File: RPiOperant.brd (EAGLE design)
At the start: 136 x 100 mm, 69 parts, among them IC1 74LS14N, IC2 74LS14N, IC3 MCP3008, J1 USB_B_PTH, J2 POWER_JACK, J3 POWER_JACK, J4 USB_B_PTH, J5 1X2-3.5MM, J6 1X2-3.5MM

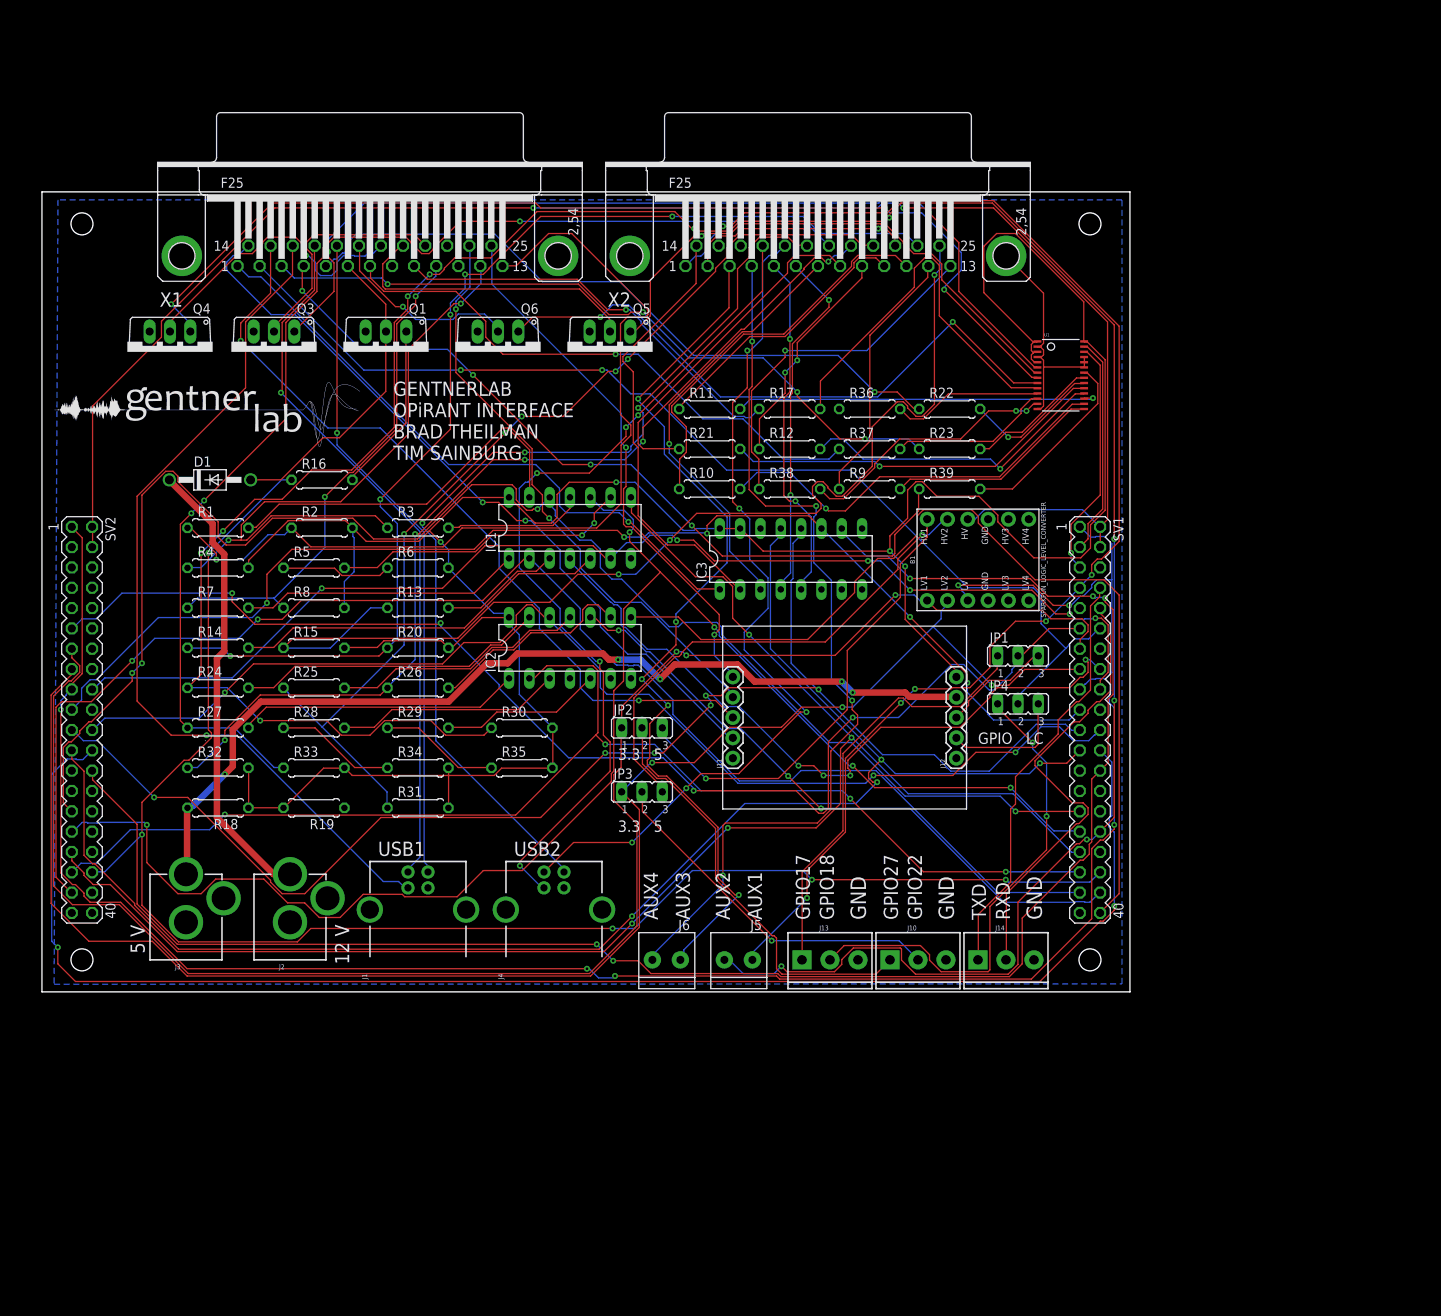
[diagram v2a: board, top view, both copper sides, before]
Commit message: alternate
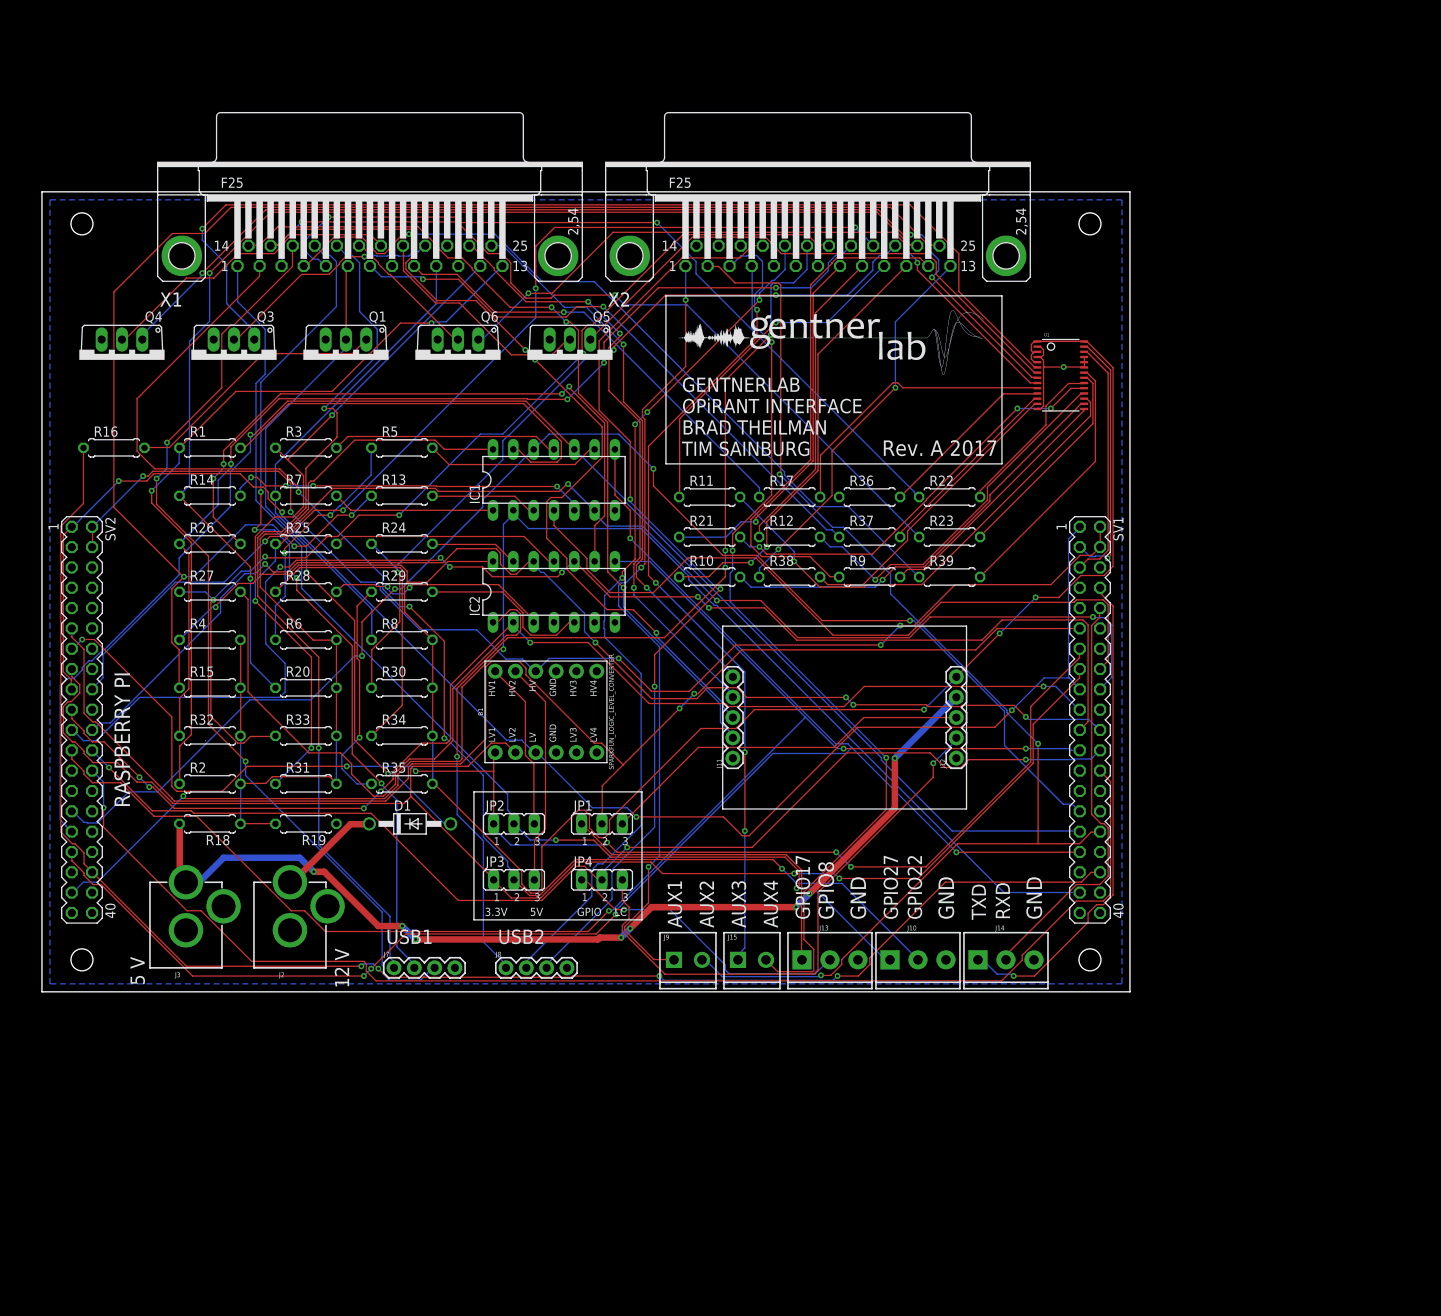
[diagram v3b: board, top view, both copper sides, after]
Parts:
- removed IC3: MCP3008, adafruit:DIL16
- removed J1, J4: USB_B_PTH, SparkFun-Connectors:USB-B-PTH
- removed J5, J6: 1X2-3.5MM, adafruit:1X2-3.5MM
- added J15, J9: (no value), SparkFun-Connectors:SCREWTERMINAL-3.5MM-2
- added J7, J8: (no value), SparkFun-Connectors:1X04
- moved B1 57.2 mm to (63.0, 35.0)
- moved JP4 56.5 mm to (70.0, 14.0)
- moved JP1 56.1 mm to (70.0, 21.0)
- moved D1 49.7 mm to (46.0, 21.0)
- moved R2 34.9 mm to (21.0, 26.0)
- moved R26 31.6 mm to (21.0, 56.0)
- moved R24 29.2 mm to (45.0, 56.0)
- moved R16 26.3 mm to (9.00, 68.0)
- moved JP2 20.0 mm to (59.0, 21.0)
- moved JP3 19.4 mm to (59.0, 14.0)
- moved R14 19.0 mm to (21.0, 62.0)
- moved R5 18.6 mm to (45.0, 68.0)
- moved R25 18.0 mm to (33.0, 56.0)
- moved R7 17.8 mm to (33.0, 62.0)
- moved R3 17.2 mm to (33.0, 68.0)
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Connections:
- removed net ADC0: IC3.1, X1.1
- removed net ADC1: IC3.2, X2.14
- removed net ADC2: IC3.3, X2.7
- removed net ADC3: IC3.4, X2.6
- removed net ADC4: IC3.5, X2.5
- removed net ADC5: IC3.6
- removed net ADC6: IC3.7
- removed net ADC7: IC3.8
- removed net CE0: SV1.24, SV2.24
- removed net CE1: IC3.10, SV1.26, SV2.26
- removed net GPIO18: JP4.2, SV1.12, X1.2
- removed net MISO: IC3.12, SV1.21, SV2.21
- removed net MOSI: IC3.11, SV1.19, SV2.19
- removed net SCLK: IC3.13, SV1.23, SV2.23
- new net GPIO7: SV1.26, SV2.26
- new net GPIO8: JP4.2, SV1.24, SV2.24
- new net N$25: X2.7
- new net N$31: X2.6
- new net N$34: X2.5
- new net N$35: X2.14
- net +3V3: no longer IC3.15, IC3.16
- net AUX1: now also J9.1; no longer J5.1, SV1.7
- net AUX2: now also J9.2; no longer J5.2
- net AUX3: now also J15.1; no longer J6.1
- net AUX4: now also J15.2; no longer J6.2
- net GND: now also J7.4, J8.4; no longer IC3.14, IC3.9, J1.GND, J1.SHLD1, J1.SHLD2, J4.GND, J4.SHLD1, J4.SHLD2
- net IR_4_GPIO: now also SV1.21, SV2.21; no longer SV1.38
- net IR_5_GPIO: now also SV1.23, SV2.23; no longer SV1.40
- net IR_6_GPIO: now also SV1.19, SV2.19; no longer SV1.35, SV2.35
- net TTL22: now also X1.2
- net TTL27: now also X1.1
- net USB1_D+: now also J7.3; no longer J1.D+
- net USB1_D-: now also J7.2; no longer J1.D-
- net USB1_VBUS: now also J7.1; no longer J1.VBUS
- net USB2_D+: now also J8.3; no longer J4.D+
- net USB2_D-: now also J8.2; no longer J4.D-
- net USB2_VBUS: now also J8.1; no longer J4.VBUS
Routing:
- net CE1: track 221.9 -> 0.00 mm, vias 5 -> 0
- net SCLK: track 192.7 -> 0.00 mm, vias 4 -> 0
- net CE0: track 188.1 -> 0.00 mm, vias 2 -> 0
- net MISO: track 176.3 -> 0.00 mm, vias 6 -> 0
- net GPIO7: track 0.00 -> 162.8 mm, vias 0 -> 1
- net MOSI: track 152.9 -> 0.00 mm, vias 5 -> 0
- net GPIO8: track 0.00 -> 145.0 mm, vias 0 -> 3
- net GPIO18: track 137.5 -> 0.00 mm, vias 2 -> 0
- net TTL22: track 44.6 -> 170.9 mm, vias 1 -> 4
- net IR_4_GPIO: track 79.1 -> 169.3 mm, vias 3 -> 6
- net TTL27: track 53.1 -> 140.7 mm, vias 0 -> 2
- net ADC0: track 78.4 -> 0.00 mm, vias 1 -> 0
- net IR_3: track 176.7 -> 102.3 mm, vias 7 -> 3
- net AUX1: track 169.4 -> 98.7 mm, vias 6 -> 3
- net RPI_3.3V: track 265.0 -> 197.8 mm, vias 6 -> 4
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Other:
- board text added: "3.3V 5V"
- board text added: "GPIO8"
- board text added: "RASPBERRY PI"
- board text added: "Rev. A 2017"
- board text removed: "3.3 5"
- board text removed: "GPIO18"

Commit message: final draft
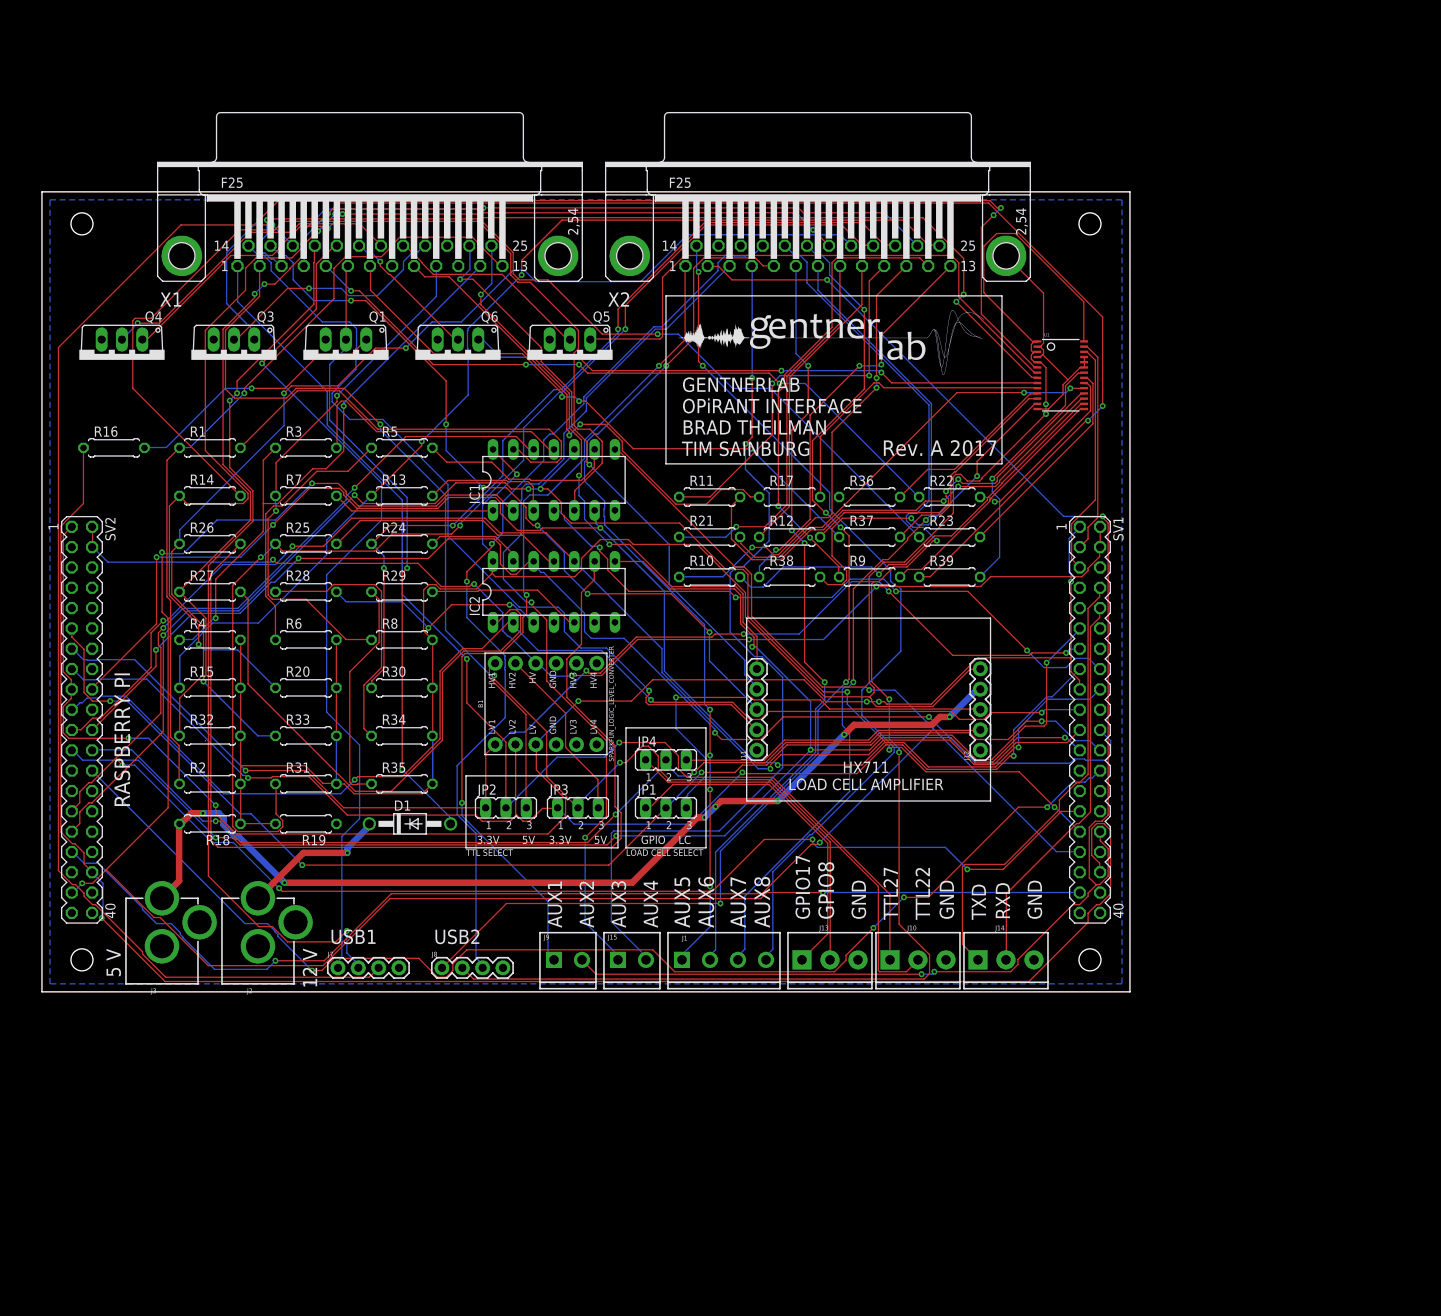
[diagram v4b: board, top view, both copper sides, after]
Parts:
- added J1: (no value), SparkFun-Connectors:SCREWTERMINAL-3.5MM-4
- moved JP4 17.0 mm to (78.0, 29.0)
- moved J15 15.0 mm to (72.0, 4.00)
- moved J9 15.0 mm to (64.0, 4.00)
- moved JP3 12.0 mm to (67.0, 23.0)
- moved JP1 8.25 mm to (78.0, 23.0)
- moved J8 8.00 mm to (50.0, 3.00)
- moved J7 7.00 mm to (37.0, 3.00)
- moved J2 4.47 mm to (27.0, -2.00)
- moved J3 3.61 mm to (15.0, -2.00)
- moved J11 3.16 mm to (89.4, 30.2)
- moved J12 3.16 mm to (117.3, 30.2)
- moved JP2 2.24 mm to (58.0, 23.0)
- moved B1 1.00 mm to (63.0, 36.0)
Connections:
- removed net N$25: X2.7
- removed net N$31: X2.6
- removed net N$34: X2.5
- removed net N$35: X2.14
- new net AUX5: J1.1, X2.5
- new net AUX6: J1.2, X2.6
- new net AUX7: J1.3, X2.7
- new net AUX8: J1.4, X2.14
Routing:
- net AUX5: track 0.00 -> 111.4 mm, vias 0 -> 5
- net AUX8: track 0.00 -> 110.5 mm, vias 0 -> 2
- net AUX7: track 0.00 -> 104.0 mm, vias 0 -> 2
- net AUX6: track 0.00 -> 95.9 mm, vias 0 -> 4
- net N$2: track 45.5 -> 122.1 mm, vias 4 -> 0
- net IR_1: track 193.6 -> 130.3 mm, vias 3 -> 2
- net USB2_D-: track 108.0 -> 170.2 mm, vias 4 -> 3
- net RGB_CUE_B: track 98.5 -> 154.0 mm, vias 1 -> 3
- net RIGHT_PECK_GPIO: track 182.0 -> 229.4 mm, vias 2 -> 4
- net HOPPER_IR_GPIO: track 173.1 -> 220.1 mm, vias 4 -> 6
- net N$5: track 84.3 -> 129.6 mm, vias 4 -> 0
- net AUX2: track 152.7 -> 188.7 mm, vias 3 -> 4
- net LCCLK: track 70.2 -> 38.4 mm, vias 1 -> 0
- net USB1_D+: track 117.5 -> 148.5 mm, vias 3 -> 1
- net +3V3: track 328.9 -> 299.4 mm
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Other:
- board text added: "AUX5"
- board text added: "AUX6"
- board text added: "AUX7"
- board text added: "AUX8"
- board text added: "HX711 LOAD CELL AMPLIFIER"
- board text added: "LOAD CELL SELECT"
- board text added: "TTL SELECT"
- board text added: "TTL22"
- board text added: "TTL27"
- board text removed: "GPIO22"
- board text removed: "GPIO27"

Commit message: Revision A
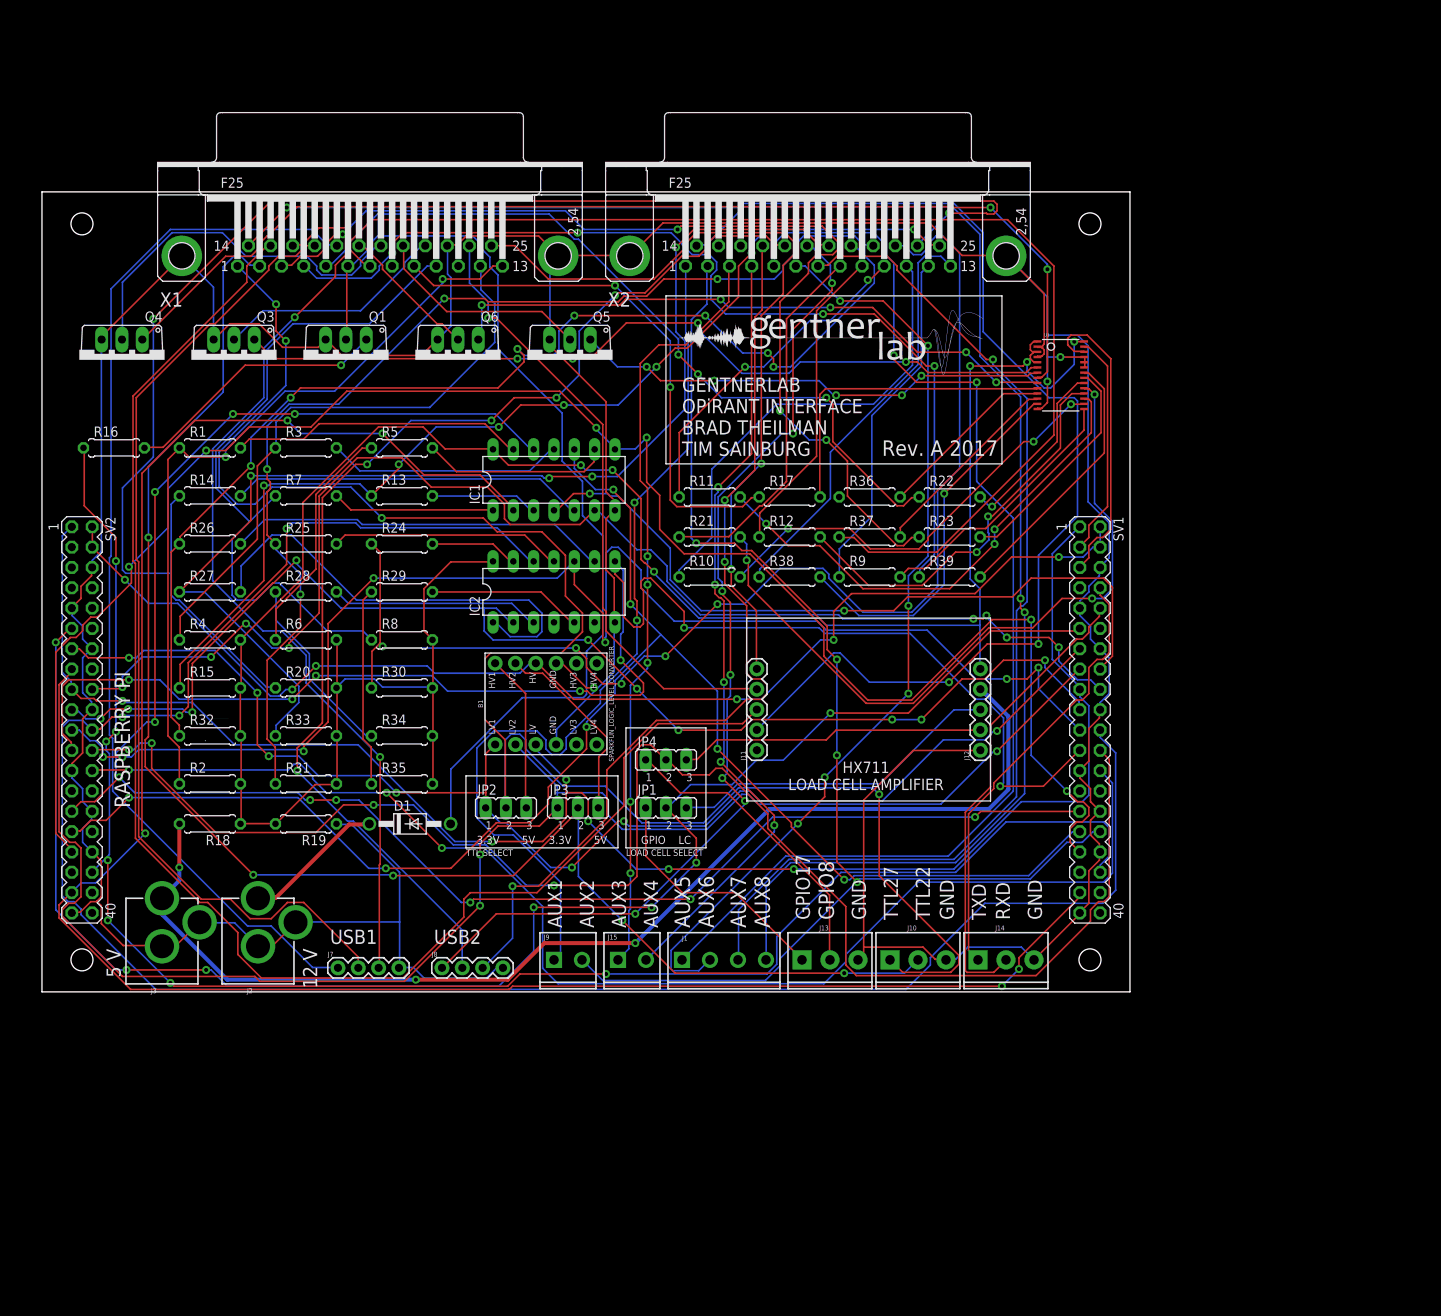
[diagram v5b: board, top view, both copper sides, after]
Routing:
- net GND: track 30.8 -> 583.7 mm, vias 0 -> 3
- net IR_3_GPIO: track 161.1 -> 262.9 mm, vias 4 -> 3
- net LOADCELLA-: track 105.3 -> 198.4 mm, vias 1 -> 3
- net LOADCELLA+: track 95.5 -> 186.8 mm, vias 6 -> 0
- net N$5: track 129.6 -> 47.7 mm
- net N$2: track 122.1 -> 44.2 mm
- net RIGHT_LED: track 74.7 -> 150.7 mm, vias 3 -> 0
- net TTL27: track 150.0 -> 223.9 mm, vias 2 -> 4
- net GPIO8: track 141.6 -> 197.8 mm
- net IR_3: track 106.9 -> 155.1 mm, vias 3 -> 5
- net AUX8: track 110.5 -> 157.4 mm
- net GPIO22: track 157.7 -> 201.1 mm
- net HOPPER: track 77.5 -> 119.4 mm, vias 2 -> 0
- net GPIO17: track 161.4 -> 199.2 mm, vias 4 -> 7
- net N$30: track 53.2 -> 90.9 mm, vias 2 -> 3
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- removed copper zone on layer 16, net GND
